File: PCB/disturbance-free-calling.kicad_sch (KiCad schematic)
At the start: 22 parts, among them U1 MOUDLE-SEEEDUINO-XIAO-ESP32C3

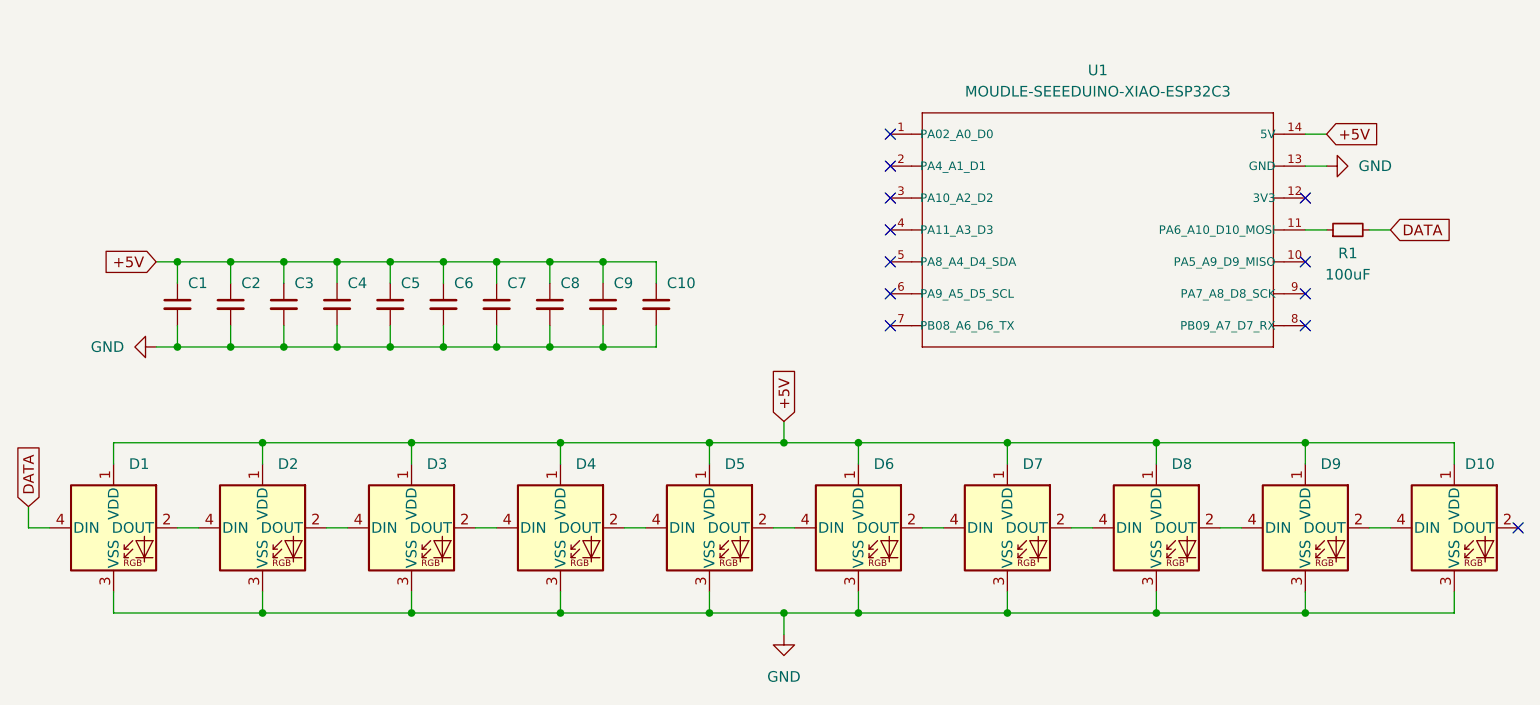
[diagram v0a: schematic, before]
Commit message: Rearrange layout
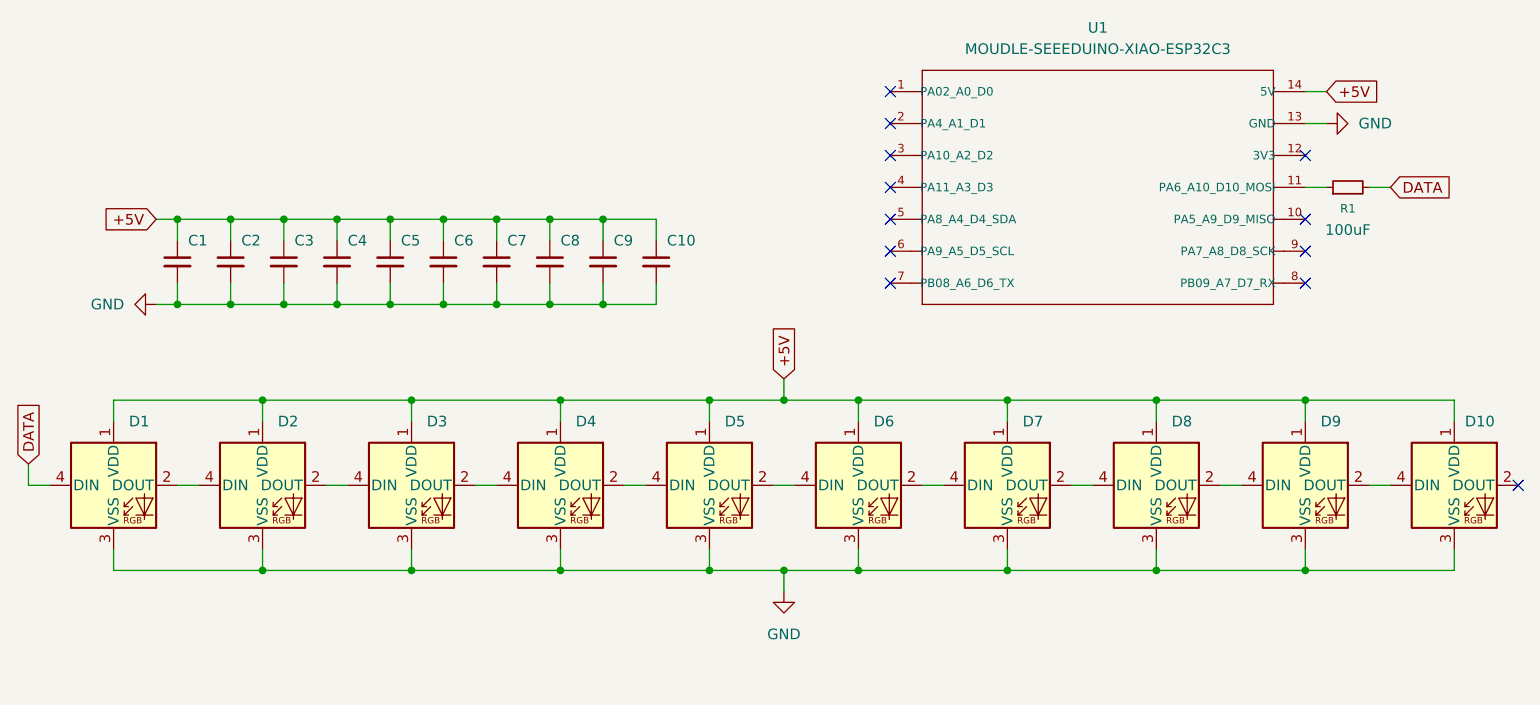
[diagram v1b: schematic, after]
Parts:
- U1: footprint MOUDLE14P-SMD-2.54-21X17.8MM -> MOUDLE-SEEEDUINO-XIAO-ESP32C3:MOUDLE14P-SMD-2.54-21X17.8MM
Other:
- title: Disturbance-Free-Calling -> Disturbance-Free Calling
- moved on the sheet: C1, C10, C2, C3, C4, C5, C6, C7, C8, C9, D1, D10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
